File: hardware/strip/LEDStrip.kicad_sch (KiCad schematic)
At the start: 4 parts, among them J201 WAGO 2065-100, J202 WAGO 2065-100, J203 WAGO 2065-100, U201 74AHC1G125

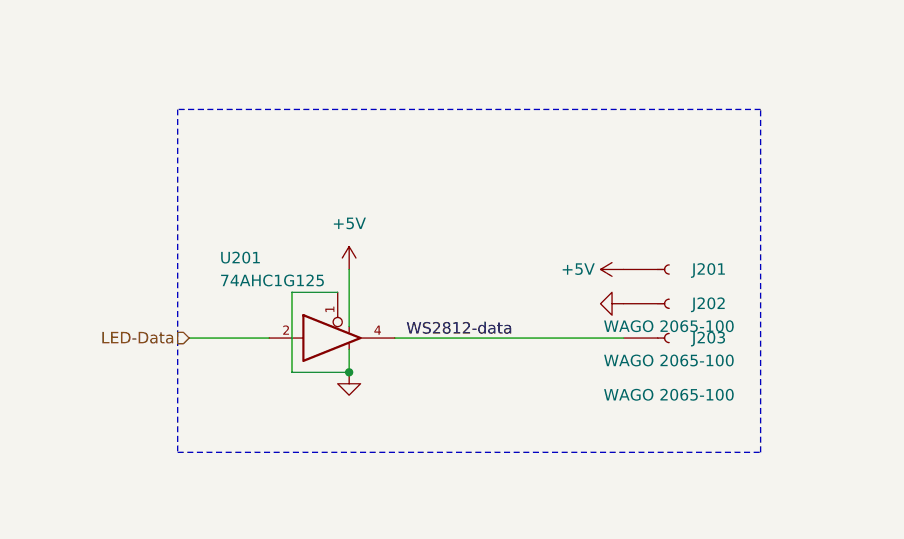
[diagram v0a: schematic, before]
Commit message: Update
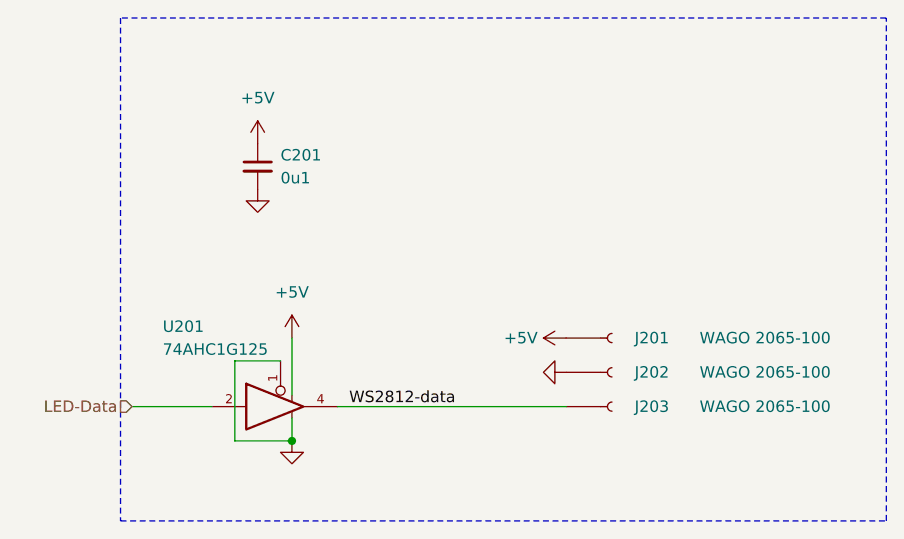
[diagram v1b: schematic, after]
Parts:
- added C201: 0u1, V2_Capacitor_SMD:C_1608, symbol V2_Capacitor:1608_0u1
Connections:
- net +5V: now also C201.1
- net GND: now also C201.2
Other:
- moved on the sheet: J201, J202, J203, U201
